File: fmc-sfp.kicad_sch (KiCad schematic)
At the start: 43 parts, among them J1 ASP-134604-01, J2 SFP+, J3 SFP+, J4 132134, J5 132134, J6 132134, J7 132134, SW1 SW_DIP_x04, U1 MAX9113EKA_TT, U2 MAX9113EKA_TT

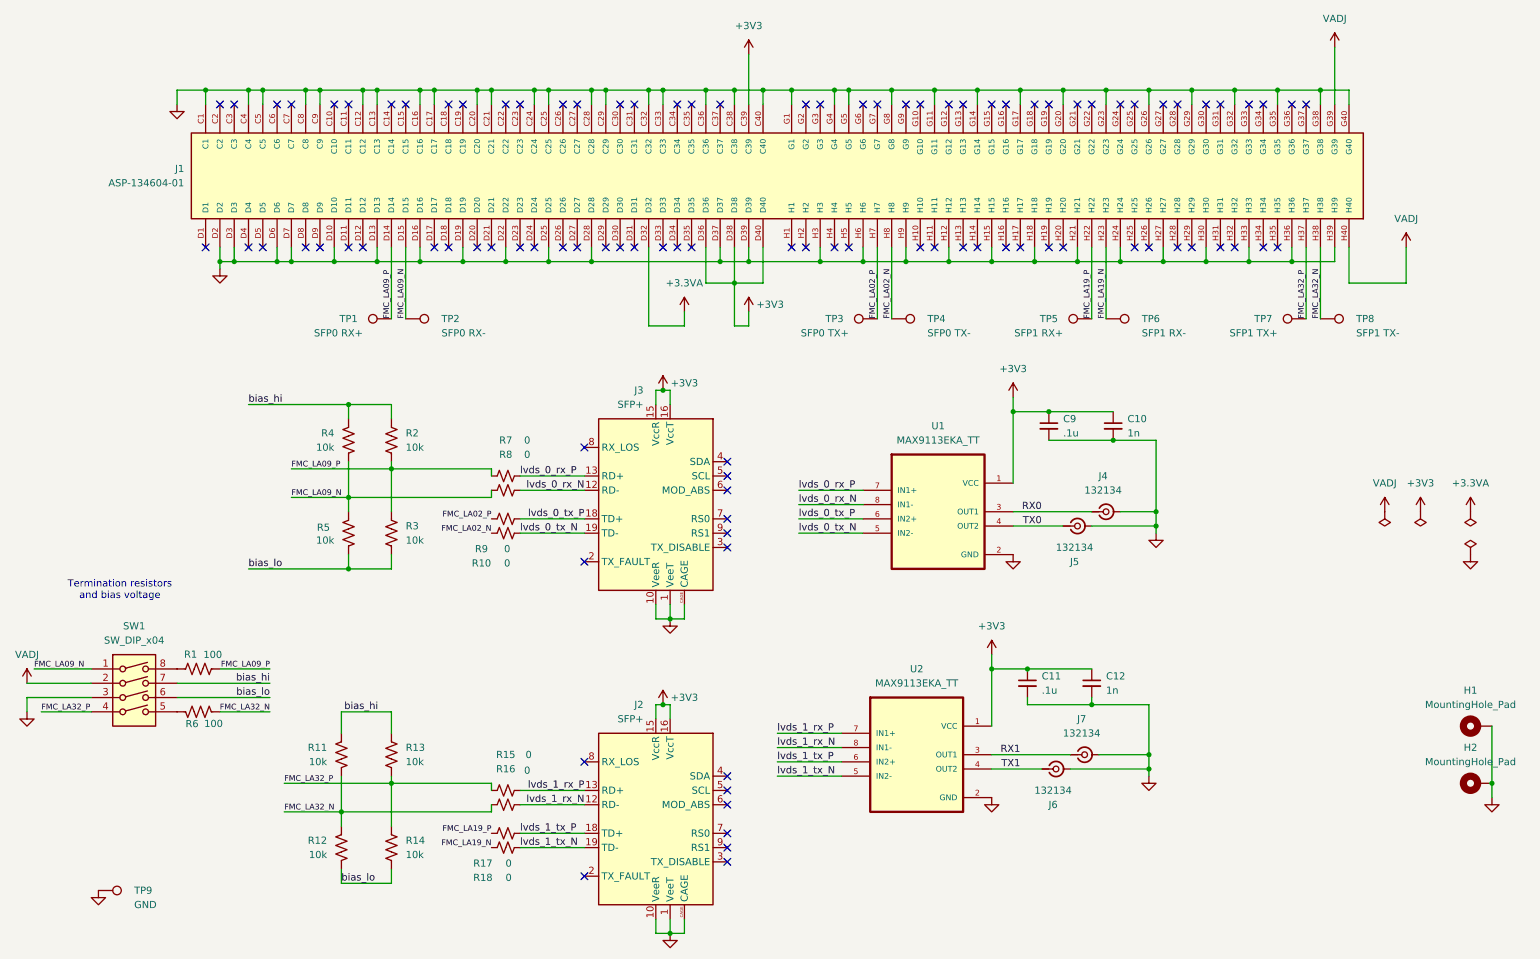
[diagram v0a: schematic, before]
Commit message: Update layout with i2c
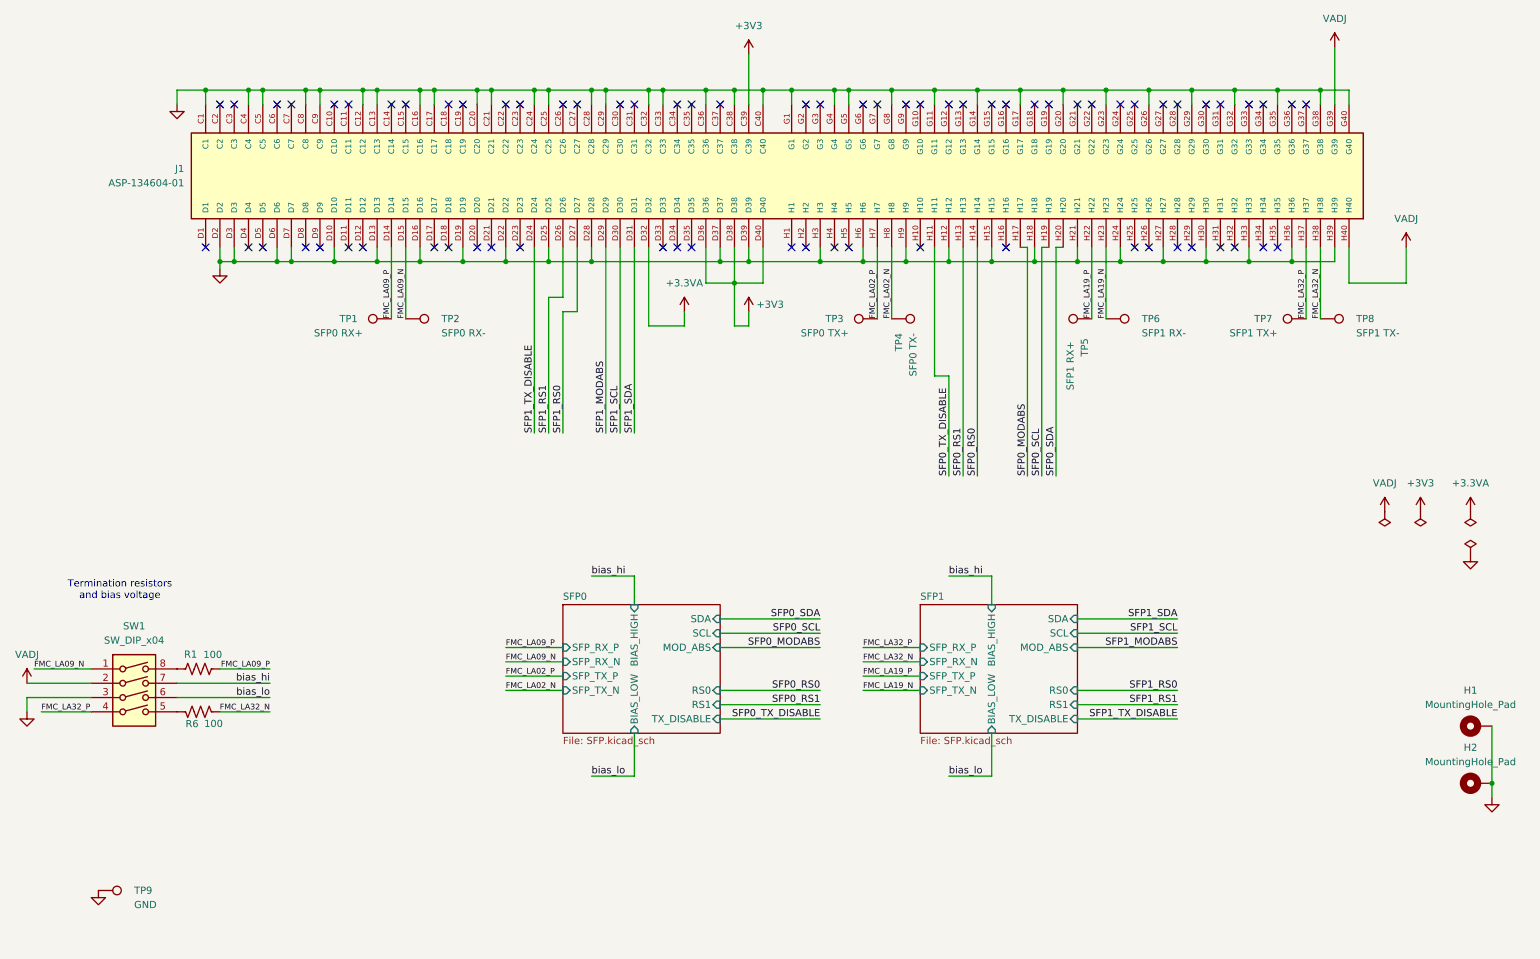
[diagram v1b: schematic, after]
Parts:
- removed C10, C12: 1n, Capacitor_SMD:C_0603_1608Metric, symbol Device:C_Small
- removed C11, C9: .1u, Capacitor_SMD:C_0603_1608Metric, symbol Device:C_Small
- removed J2, J3: SFP+, project:SFP_and_Cage, symbol Interface_Optical:SFP+
- removed J4, J5, J6, J7: 132134, Connector_Coaxial:SMA_Amphenol_132134_Vertical, symbol Connector:Conn_Coaxial_Small
- removed R10, R15, R16, R17, R18, R7, R8, R9: 0, Resistor_SMD:R_0805_2012Metric_Pad1.20x1.40mm_HandSolder, symbol Device:R_Small_US
- removed R11, R12, R13, R14, R2, R3, R4, R5: 10k, Resistor_SMD:R_0805_2012Metric_Pad1.20x1.40mm_HandSolder, symbol Device:R_US
- removed U1, U2: MAX9113EKA_TT, Package_TO_SOT_SMD:SOT-23-8, symbol project:MAX9113EKA_TT
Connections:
- net SFP1_TX_DISABLE: now reaches J1.D24
- net SFP1_RS1: now reaches J1.D26
- net SFP1_RS0: now reaches J1.D27
- net SFP1_MODABS: now reaches J1.D29
- net SFP1_SCL: now reaches J1.D30
- net SFP1_SDA: now reaches J1.D31
- net SFP0_TX_DISABLE: now reaches J1.H11
- net SFP0_RS1: now reaches J1.H13
- net SFP0_RS0: now reaches J1.H14
- net SFP0_MODABS: now reaches J1.H17
- net SFP0_SCL: now reaches J1.H19
- net SFP0_SDA: now reaches J1.H20
- no-connect marks 100 -> 72
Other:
- added sheet SFP0 (SFP.kicad_sch)
- added sheet SFP1 (SFP.kicad_sch)
